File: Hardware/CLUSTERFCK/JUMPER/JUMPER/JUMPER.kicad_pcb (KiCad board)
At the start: 2 copper layers, 142 x 53.3 mm, 2 parts, among them J1 Conn_02x20_Counter_Clockwise, J2 Conn_02x20_Counter_Clockwise

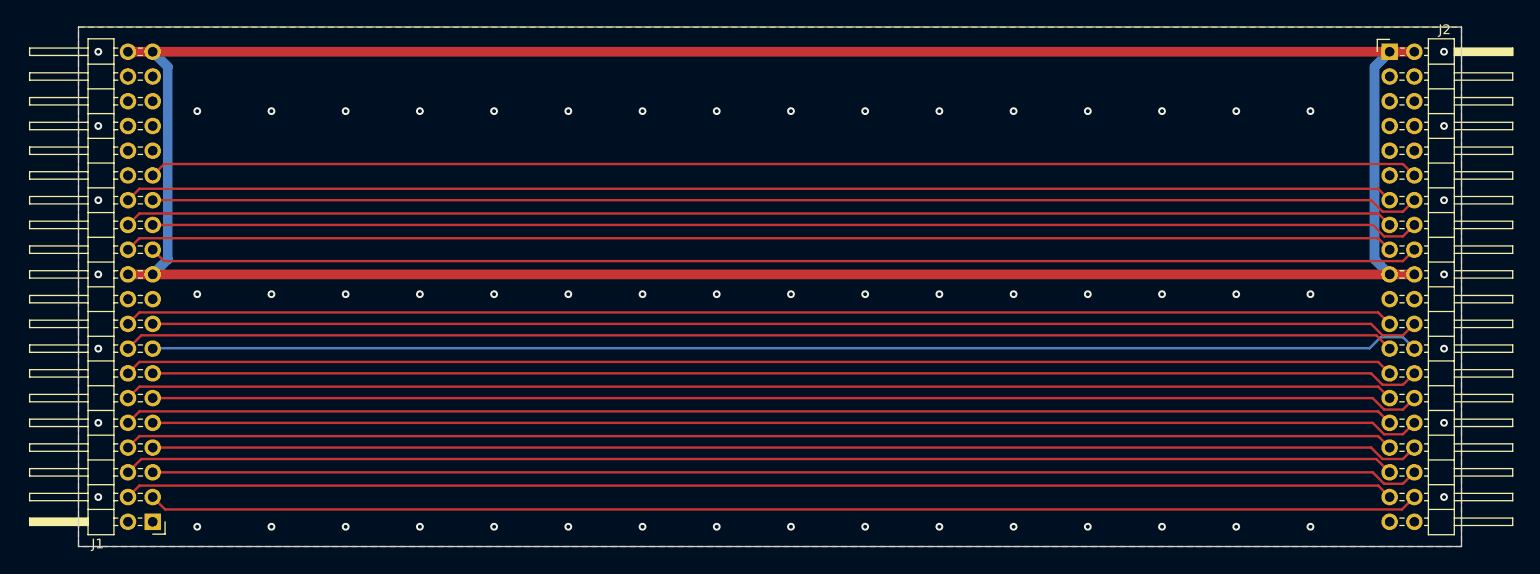
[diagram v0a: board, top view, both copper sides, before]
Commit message: 0059 | 0,5h | Review JUMPER
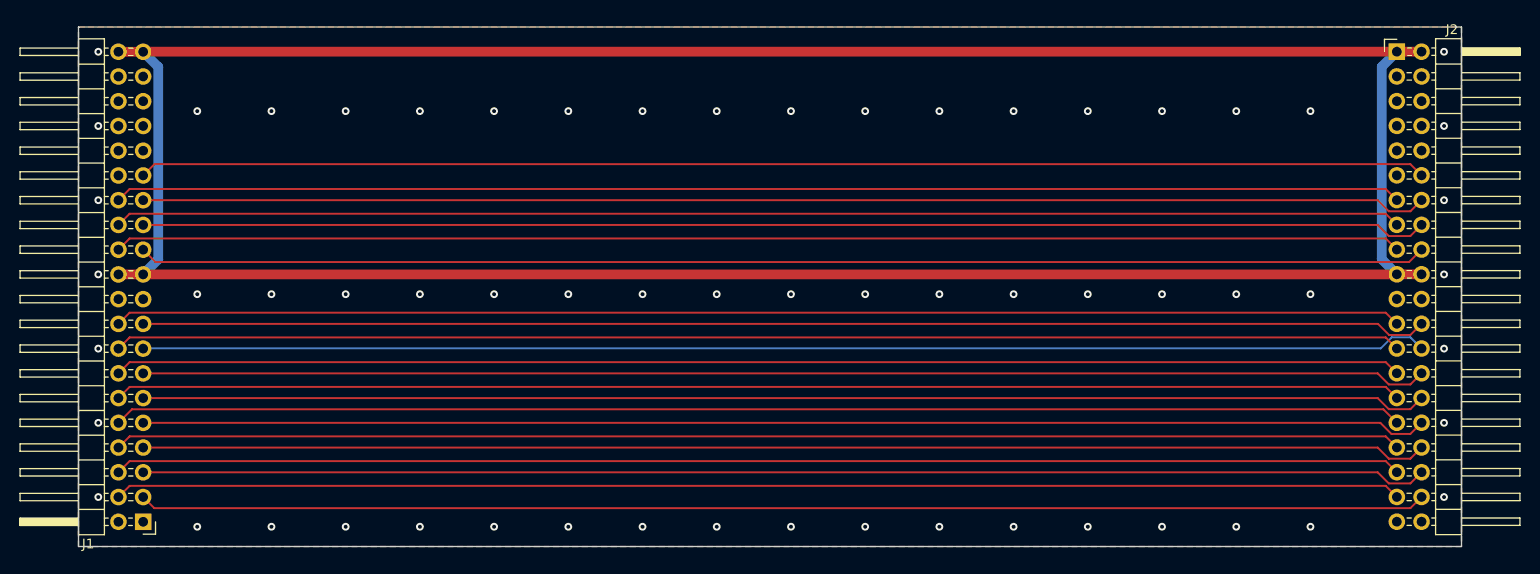
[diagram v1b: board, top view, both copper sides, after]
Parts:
- moved J1 0.98 mm to (6.64, 50.8)
- moved J2 0.74 mm to (135.4, 2.53)
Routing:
- net +5V: track 312.4 -> 315.9 mm
- net /ADDR7: track 130.5 -> 132.4 mm
- net EXT2: track 130.5 -> 132.3 mm
- net zero: track 130.5 -> 132.2 mm
- net CLK: track 130.5 -> 132.2 mm
- net ~BI: track 130.5 -> 132.2 mm
- net /ADDR6: track 130.5 -> 132.2 mm
- net /ADDR2: track 130.5 -> 132.2 mm
- net /ADDR10: track 130.5 -> 132.2 mm
- net ~AI: track 130.5 -> 132.2 mm
- net carry: track 130.5 -> 132.2 mm
- net SU: track 130.5 -> 132.2 mm
- net EXT1: track 130.5 -> 132.2 mm
- net EXT0: track 130.5 -> 132.2 mm
- net /ADDR9: track 130.5 -> 132.2 mm
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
